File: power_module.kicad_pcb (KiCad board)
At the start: 2 copper layers, 33 parts, among them J1 USB_B, J2 VOUT, J3 CONN_01X03, J4 CONN_01X06, J5 CONN_01X02, J6 CONN_01X02, Q1 Q_NMOS_GSD, U1 ATTINY24A-SSU

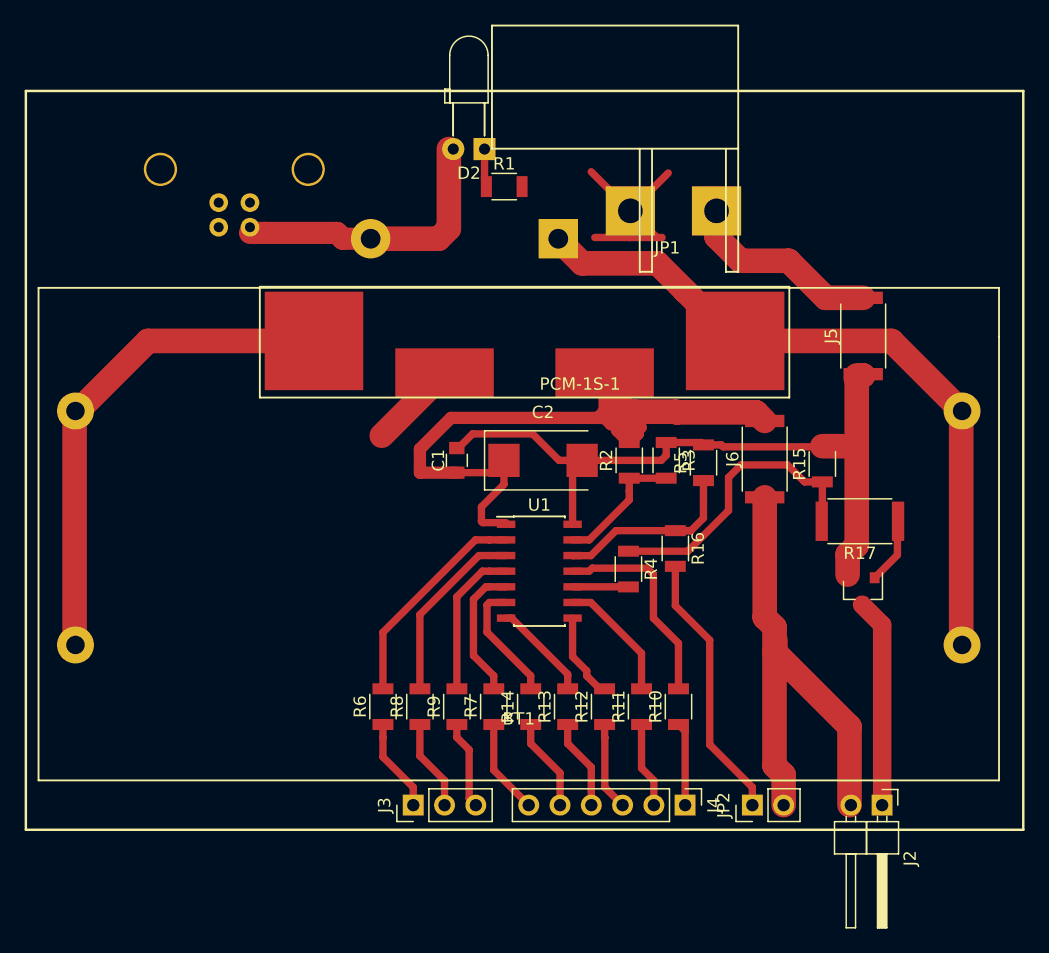
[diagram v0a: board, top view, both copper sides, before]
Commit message: Мелкие поправки по плате
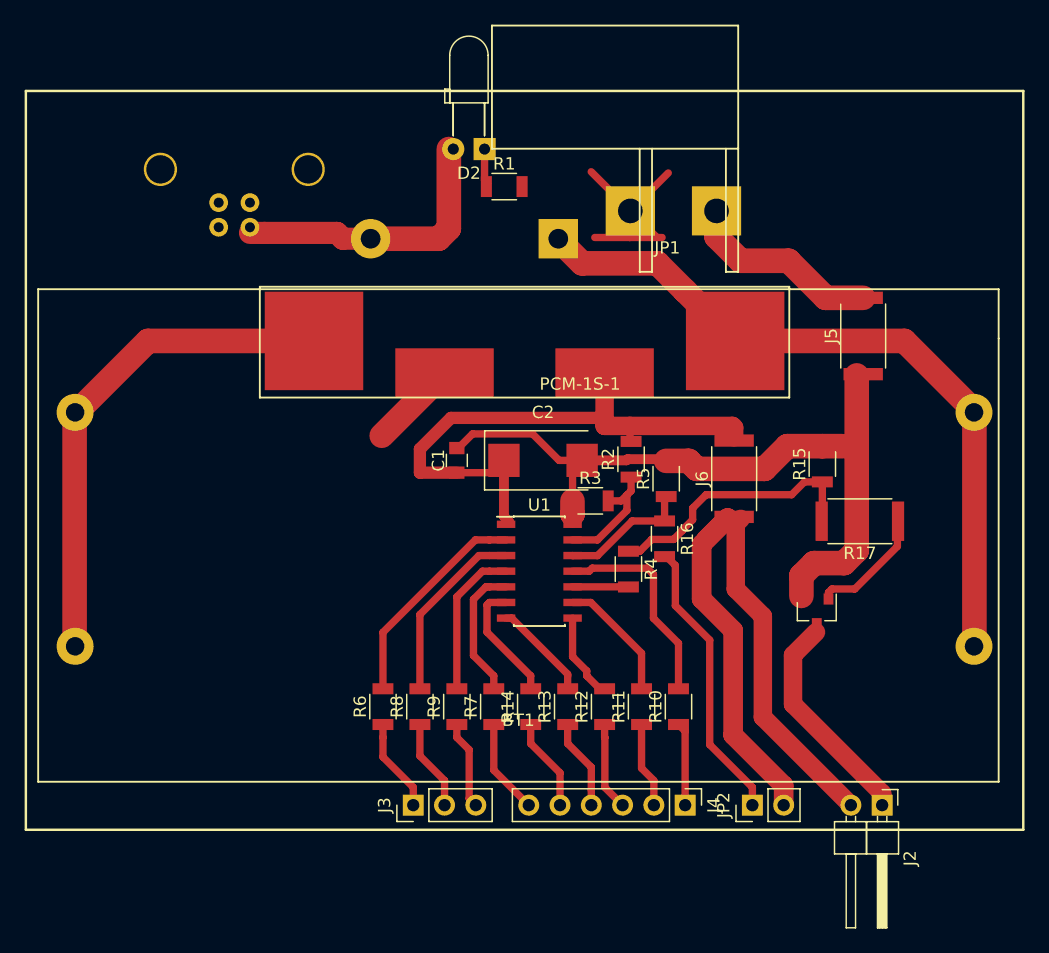
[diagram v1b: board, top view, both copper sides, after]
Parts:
- BT1: footprint BH-18650-PC4 -> BH-18650-PC4:BH-18650-PC4
- moved R3 6.98 mm to (230.8, 58.3), turned to 0 degrees
- moved Q1 4.13 mm to (249.2, 67.3)
- moved R5 3.30 mm to (237.0, 56.5)
- moved J6 2.95 mm to (242.5, 56.5)
- moved R16 1.18 mm to (236.9, 61.4)
- moved R2 0.17 mm to (234.2, 54.9)
- moved BT1 0.11 mm to (225.0, 61.1)
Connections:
- net Net-(J3-Pad1) renamed /led.green
- R14 pad 2: /ss -> Net-(R14-Pad2)
- R7 pad 2: Net-(R7-Pad2) -> /ss
- U1 pad 5: Net-(R7-Pad2) -> /ss
- U1 pad 6: /ss -> Net-(R14-Pad2)
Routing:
- net Net-(R7-Pad2): track 11.0 -> 0.00 mm
- net Net-(R14-Pad2): track 0.00 -> 9.91 mm
- net /pwr_btn: track 16.2 -> 10.7 mm
- net Net-(Q1-Pad1): track 5.61 -> 9.97 mm
- net GNDA: track 75.0 -> 77.7 mm
- net +4V: track 105.0 -> 107.6 mm
- net Net-(R15-Pad1): track 23.1 -> 21.0 mm
- net Net-(J2-Pad1): track 17.0 -> 18.5 mm
- net /ss: track 9.91 -> 11.0 mm
- net Net-(JP2-Pad1): track 22.0 -> 23.1 mm
- net Net-(BT1-Pad1): track 57.6 -> 58.6 mm
- net Net-(R2-Pad1): track 10.7 -> 9.83 mm
